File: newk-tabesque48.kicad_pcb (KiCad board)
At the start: 2 copper layers, 192.5 x 118.4 mm, 98 parts, among them SW1 SW_Push, U1 ProMicro

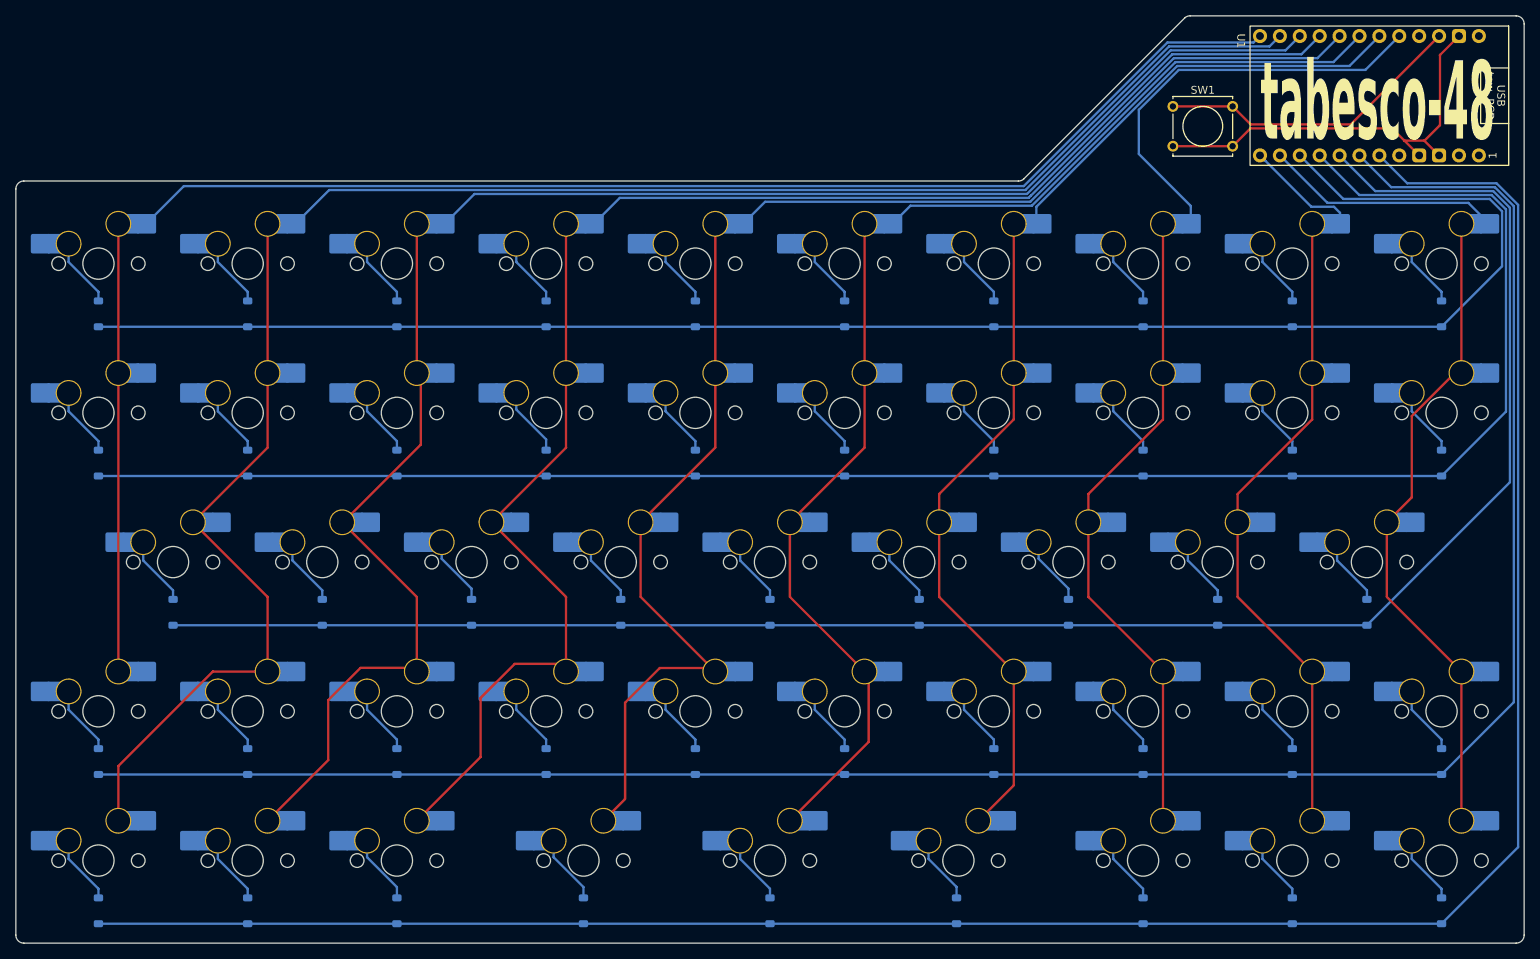
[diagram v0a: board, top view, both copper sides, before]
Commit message: 5u
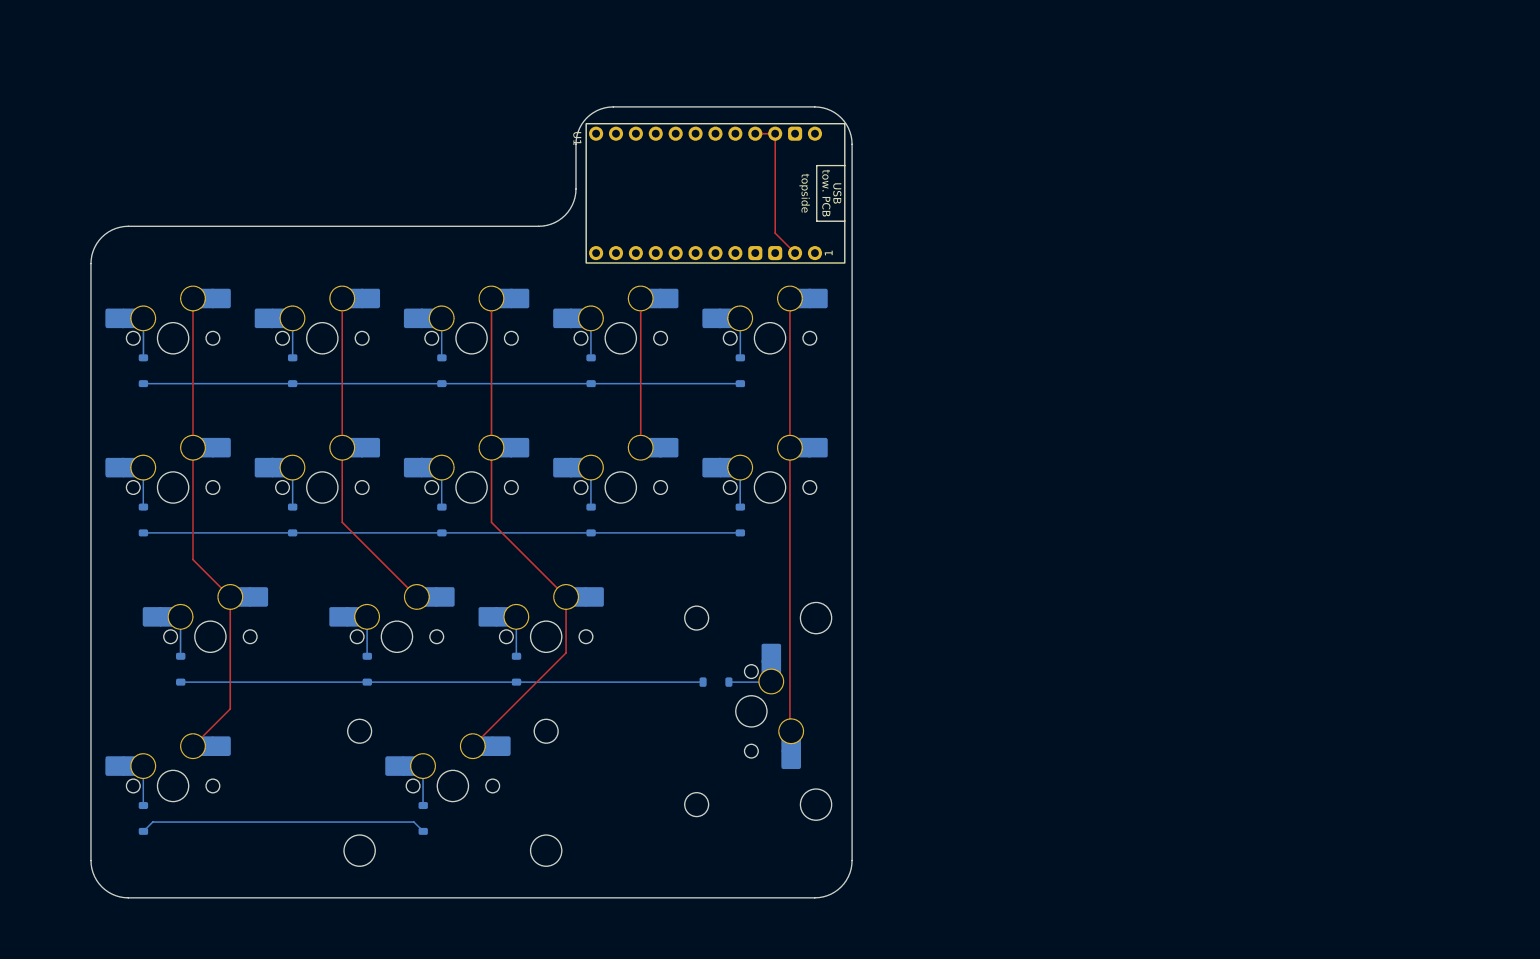
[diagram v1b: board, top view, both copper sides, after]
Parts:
- removed D17, D18, D19, D20, D21, D22, D23, D24, D25, D26, D27, D28, D29, D30, D31, D32, D33, D34, D35, D36, D37, D38, D39, D40, D41, D42, D43, D44, D45, D46, D47, D48: D_Small, Diode_SMD:D_SOD-123
- removed MX17, MX18, MX19, MX20, MX21, MX22, MX23, MX24, MX25, MX26, MX27, MX28, MX29, MX30, MX31, MX32, MX33, MX34, MX35, MX36, MX37, MX38, MX39, MX40, MX41, MX42, MX43, MX44, MX45, MX46, MX47, MX48: MX_SW_HS, marbastlib-mx:SW_MX_HS_CPG151101S11_1u
- removed SW1: SW_Push, Button_Switch_THT:SW_Tactile_Straight_KSA0Axx1LFTR
- added REF**: STAB_MX_2.75u, marbastlib-mx:STAB_MX_2.75u, F.Cu at (114.7, 124.6)
- added REF**: STAB_MX_ISO, marbastlib-mx:STAB_MX_ISO, F.Cu at (152.8, 115.1)
- moved D1 165.9 mm to (75.2, 71.6)
- moved D11 163.1 mm to (80.0, 109.7)
- moved MX1 162.2 mm to (79.0, 67.4)
- moved MX11 159.7 mm to (83.8, 105.5)
- moved D2 127.8 mm to (94.3, 71.6)
- moved MX2 124.2 mm to (98.0, 67.4)
- moved D12 121.0 mm to (103.8, 109.7)
- moved MX12 117.8 mm to (107.6, 105.5)
- moved D15 100.3 mm to (75.2, 128.7)
- moved MX15 98.1 mm to (79.0, 124.6)
- moved MX10 90.4 mm to (155.2, 86.5)
- moved D3 89.8 mm to (113.3, 71.6)
- moved MX3 86.2 mm to (117.1, 67.4)
- moved D10 86.1 mm to (151.4, 90.6)
- moved U1 85.7 mm to (147.0, 48.9)
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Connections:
- D10 pad 1: /row0 -> /row1
- D11 pad 1: /row1 -> /row2
- D12 pad 1: /row1 -> /row2
- D13 pad 1: /row1 -> /row2
- D14 pad 1: /row1 -> /row2
- D15 pad 1: /row1 -> /row3
- D16 pad 1: /row1 -> /row3
- D6 pad 1: /row0 -> /row1
- D7 pad 1: /row0 -> /row1
- D8 pad 1: /row0 -> /row1
- D9 pad 1: /row0 -> /row1
- MX10 pad 2: /col9 -> /col4
- MX14 pad 2: /col3 -> /col4
- MX15 pad 2: /col4 -> /col0
- MX16 pad 2: /col5 -> /col2
- MX6 pad 2: /col5 -> /col0
- MX7 pad 2: /col6 -> /col1
- MX8 pad 2: /col7 -> /col2
- MX9 pad 2: /col8 -> /col3
- U1 pad 10: /row0 -> unconnected-(U1-E6-Pad10)
- U1 pad 11: /col0 -> unconnected-(U1-B4-Pad11)
- U1 pad 12: /col1 -> unconnected-(U1-B5-Pad12)
- U1 pad 15: RST -> unconnected-(U1-RST-Pad15)
- U1 pad 17: /col2 -> unconnected-(U1-F4-Pad17)
- U1 pad 18: /col3 -> unconnected-(U1-F5-Pad18)
- U1 pad 19: /col4 -> unconnected-(U1-F6-Pad19)
- U1 pad 20: /col5 -> unconnected-(U1-F7-Pad20)
- U1 pad 21: /col6 -> unconnected-(U1-B1-Pad21)
- U1 pad 22: /col7 -> unconnected-(U1-B3-Pad22)
- U1 pad 23: /col8 -> unconnected-(U1-B2-Pad23)
- U1 pad 24: /col9 -> unconnected-(U1-B6-Pad24)
- U1 pad 5: /col_tmo -> unconnected-(U1-D1-Pad5)
- U1 pad 6: /row4 -> unconnected-(U1-D0-Pad6)
- U1 pad 7: /row3 -> unconnected-(U1-D4-Pad7)
- U1 pad 8: /row2 -> unconnected-(U1-C6-Pad8)
- U1 pad 9: /row1 -> unconnected-(U1-D7-Pad9)
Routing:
- net /row4: track 287.6 -> 0.00 mm
- net /col8: track 235.2 -> 0.00 mm
- net /row3: track 270.2 -> 36.7 mm
- net /col7: track 220.0 -> 0.00 mm
- net /col9: track 212.8 -> 0.00 mm
- net /col6: track 203.3 -> 0.00 mm
- net /col5: track 184.4 -> 0.00 mm
- net /row2: track 237.8 -> 66.7 mm
- net /row1: track 235.5 -> 76.2 mm
- net /row0: track 218.2 -> 76.2 mm
- net /col3: track 141.2 -> 19.1 mm
- net /col4: track 161.6 -> 55.3 mm
- net /col2: track 138.5 -> 66.0 mm
- net /col1: track 98.8 -> 42.0 mm
- net /col0: track 114.9 -> 61.1 mm
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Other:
- board size 192.5 x 118.4 mm -> 97.2 x 101 mm
- board text removed: "here's some keys to copy and paste since they're not on this keyboard: tab esc backspace capslock ` ~ - _ = + [ { ] } ; : ' {dblquote} \ | , < . > / ? f1 f2 f3 f4 f5 f6 f7 f8 f9 f10 f11 f12 Rshift Ralt Rsuper menu Rctrl printscr scroll lock pause insert home pgup delete end pgdown numlock"
- board text removed: "tabesco-48"
